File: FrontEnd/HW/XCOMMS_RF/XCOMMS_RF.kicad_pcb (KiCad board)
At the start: 2 copper layers, 40 x 65 mm, 82 parts, among them J1 SMA, J2 SMA, J3 SFC-110-T2-F-D-A-TR, U1 SIM-14+, U2 HMC788ALP2ETR, U3 HMC952ALP5GE, U4 LMX2572RHAT, U5 HMC788ALP2ETR, U6 AD8031, U7 ADT7310, Y1 TCXO 25 MHz

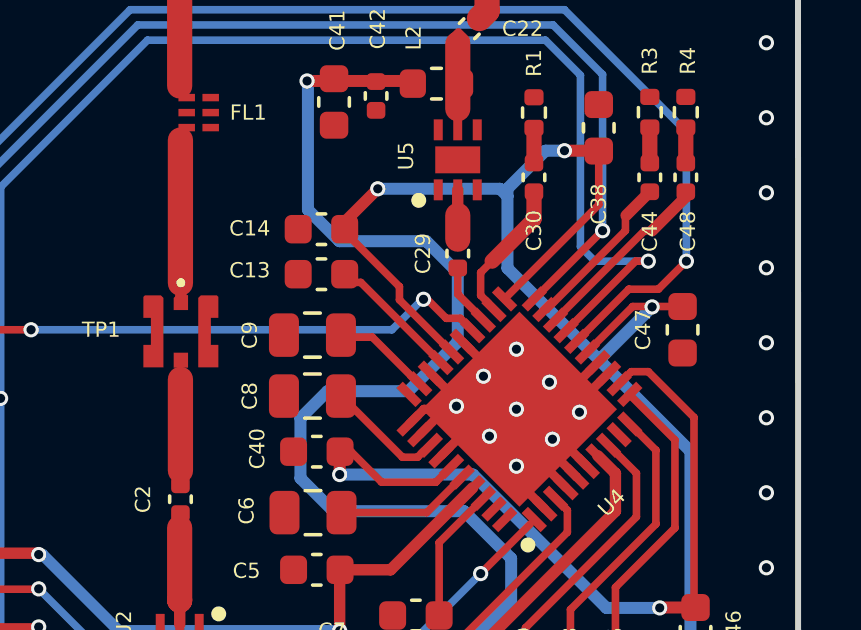
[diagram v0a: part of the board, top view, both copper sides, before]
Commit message: changes
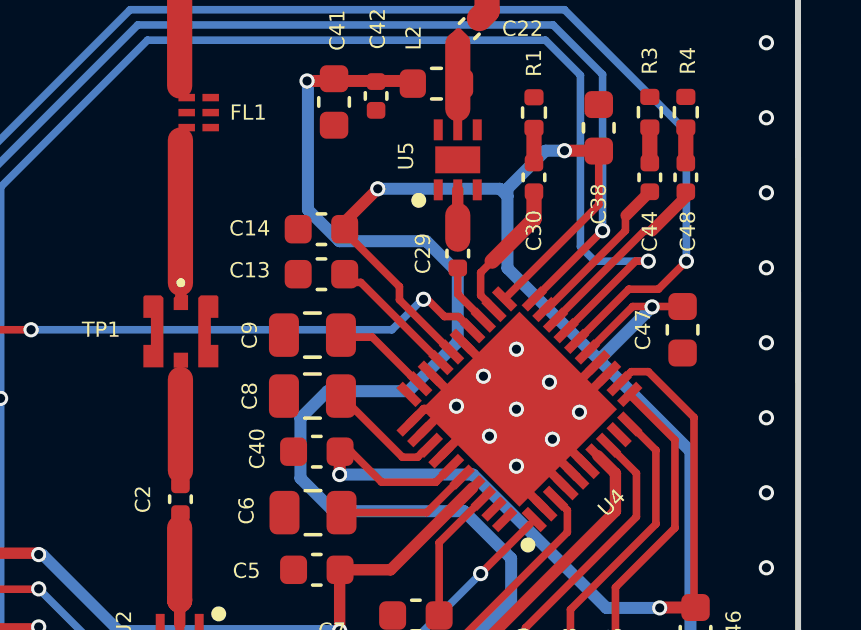
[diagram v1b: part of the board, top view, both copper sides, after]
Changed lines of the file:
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@@
     (fp_line (start -0.14058 0.51) (end 0.14058 0.51) (layer "F.SilkS") (width 0.12))
     (fp_line (start -0.14058 -0.51) (end 0.14058 -0.51) (layer "F.SilkS") (width 0.12))
+    (fp_line (start -1.48 -0.73) (end 1.48 -0.73) (layer "F.CrtYd") (width 0.05))
     (fp_line (start -1.48 0.73) (end -1.48 -0.73) (layer "F.CrtYd") (width 0.05))
-    (fp_line (start 1.48 -0.73) (end 1.48 0.73) (layer "F.CrtYd") (width 0.05))
     (fp_line (start 1.48 0.73) (end -1.48 0.73) (layer "F.CrtYd") (width 0.05))
-    (fp_line (start -1.48 -0.73) (end 1.48 -0.73) (layer "F.CrtYd") (width 0.05))
+    (fp_line (start 1.48 -0.73) (end 1.48 0.73) (layer "F.CrtYd") (width 0.05))
     (fp_line (start -0.8 0.4) (end -0.8 -0.4) (layer "F.Fab") (width 0.1))
-    (fp_line (start -0.8 -0.4) (end 0.8 -0.4) (layer "F.Fab") (width 0.1))
     (fp_line (start 0.8 -0.4) (end 0.8 0.4) (layer "F.Fab") (width 0.1))
+    (fp_line (start -0.8 -0.4) (end 0.8 -0.4) (layer "F.Fab") (width 0.1))
     (fp_line (start 0.8 0.4) (end -0.8 0.4) (layer "F.Fab") (width 0.1))
     (pad "1" smd roundrect (at -0.775 0 270) (size 0.9 0.95) (layers "F.Cu" "F.Paste" "F.Mask") (roundrect_rratio 0.25)
@@
   (segment (start 147.420998 96.452) (end 144.626998 96.452) (width 0.254) (layer "F.Cu") (net 14))
   (segment (start 140.816998 92.642) (end 140.308998 92.642) (width 0.254) (layer "F.Cu") (net 14))
-  (segment (start 160.62623 95.436) (end 161.26123 96.071) (width 0.254) (layer "F.Cu") (net 14))
-  (segment (start 161.26123 96.071) (end 161.731669 96.071) (width 0.254) (layer "F.Cu") (net 14))
-  (segment (start 144.626998 96.452) (end 140.816998 92.642) (width 0.254) (layer "F.Cu") (net 14))
-  (segment (start 161.731669 96.071) (end 162.144375 96.483706) (width 0.254) (layer "F.Cu") (net 14))
+  (segment (start 161.20223 96.012) (end 161.672669 96.012) (width 0.254) (layer "F.Cu") (net 14))
+  (segment (start 160.62623 95.436) (end 161.20223 96.012) (width 0.254) (layer "F.Cu") (net 14))
   (segment (start 160.501998 95.436) (end 160.62623 95.436) (width 0.254) (layer "F.Cu") (net 14))
+  (segment (start 144.626998 96.452) (end 140.816998 92.642) (width 0.254) (layer "F.Cu") (net 14))
+  (segment (start 161.672669 96.012) (end 162.144375 96.483706) (width 0.254) (layer "F.Cu") (net 14))
   (via (at 160.501998 95.436) (size 0.508) (drill 0.3048) (layers "F.Cu" "B.Cu") (net 14))
   (via (at 140.308998 92.642) (size 0.508) (drill 0.3048) (layers "F.Cu" "B.Cu") (net 14))
